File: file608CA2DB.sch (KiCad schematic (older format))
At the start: 1 part, among them SW5 SW_SP3T

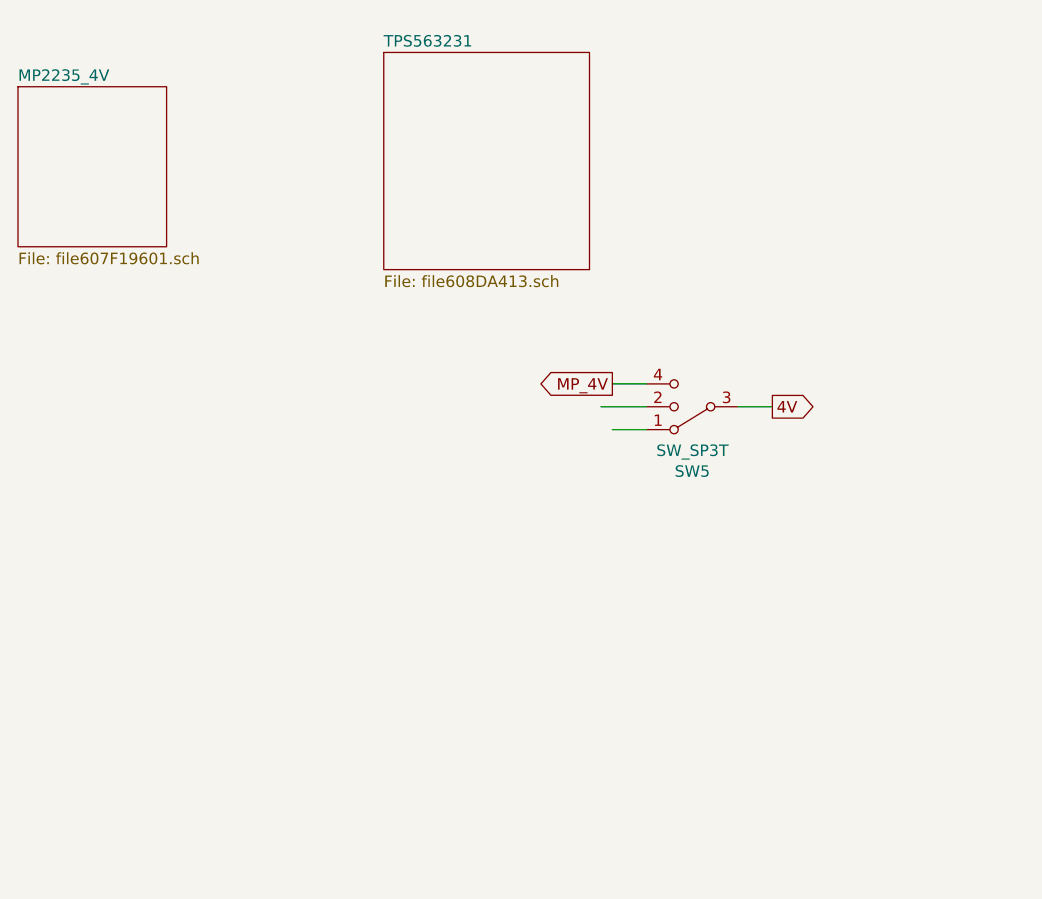
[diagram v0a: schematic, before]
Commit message: full schematic, version 1.0
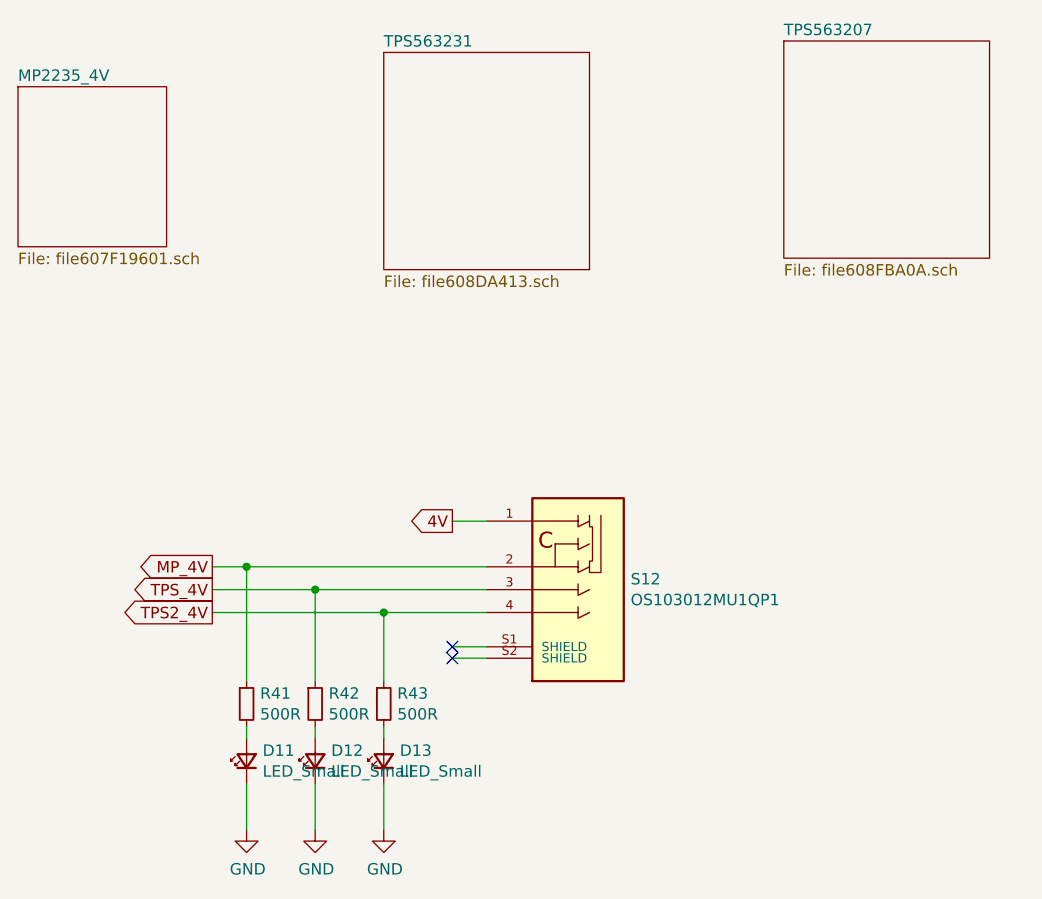
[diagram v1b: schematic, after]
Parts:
- removed SW5: SW_SP3T, symbol Switch:SW_SP3T
- added D11, D12, D13: LED_Small, Diode_SMD:D_0603_1608Metric_Pad1.05x0.95mm_HandSolder, symbol Device:LED_Small
- added R41, R42, R43: 500R, Resistor_SMD:R_0805_2012Metric_Pad1.20x1.40mm_HandSolder, symbol Device:R_Small
- added S12: OS103012MU1QP1, EIPP:SW_OS103012MU1QP1, symbol EIPP_LIBRARY:OS103012MU1QP1
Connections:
- net labels added: GND, TPS2_4V, TPS_4V
- wire segments 4 -> 18
- no-connect marks 0 -> 2
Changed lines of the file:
@@
 $Descr A4 11693 8268
 encoding utf-8
-Sheet 8 10
+Sheet 8 15
 Title ""
 Date ""
@@
 Comment4 ""
 $EndDescr
-$Comp
-L Switch:SW_SP3T SW?
-U 1 1 608CBBC4
-P 5500 3200
-AR Path="/607D64D2/608CBBC4" Ref="SW?"  Part="1"
-AR Path="/608CA2DC/608CBBC4" Ref="SW5"  Part="1"
-F 0 "SW5" H 5500 3483 50  0000 C CNN
-F 1 "SW_SP3T" H 5500 3392 50  0000 C CNN
-F 2 "" H 4875 3375 50  0001 C CNN
-F 3 "~" H 4875 3375 50  0001 C CNN
-	1    5500 3200
-	-1   0    0    1
-$EndComp
-Wire Wire Line
-	5150 3100 5300 3100
-Wire Wire Line
-	5300 3200 5100 3200
-Wire Wire Line
-	5300 3300 5150 3300
-Wire Wire Line
-	5700 3200 5850 3200
-Text GLabel 5850 3200 2    50   Output ~ 0
+Wire Wire Line
+	4600 3700 4450 3700
+Text GLabel 4450 3700 0    50   Output ~ 0
 4V
-Text GLabel 5150 3100 0    50   Output ~ 0
+Text GLabel 3400 3900 0    50   Output ~ 0
 MP_4V
 $Sheet
@@
 F1 "file608DA413.sch" 50
 $EndSheet
+Text GLabel 3400 4000 0    50   Output ~ 0
+TPS_4V
+$Sheet
+S 5900 1600 900  950
+U 608FBA0B
+F0 "TPS563207" 50
+F1 "file608FBA0A.sch" 50
+$EndSheet
+Text GLabel 3400 4100 0    50   Output ~ 0
+TPS2_4V
+$Comp
+L EIPP_LIBRARY:OS103012MU1QP1 S12
+U 1 1 608FBF88
+P 5000 4000
+F 0 "S12" H 5230 4046 50  0000 L CNN
+F 1 "OS103012MU1QP1" H 5230 3955 50  0000 L CNN
+F 2 "EIPP:SW_OS103012MU1QP1" H 5000 4000 50  0001 L BNN
+F 3 "" H 5000 4000 50  0001 L BNN
+F 4 "9.2 mm" H 5000 4000 50  0001 L BNN "MAXIMUM_PACKAGE_HEIGHT"
+F 5 "C and K Switches" H 5000 4000 50  0001 L BNN "MANUFACTURER"
+F 6 "Manufacturer Recommendations" H 5000 4000 50  0001 L BNN "STANDARD"
+F 7 "8 Aug 17" H 5000 4000 50  0001 L BNN "PARTREV"
+	1    5000 4000
+	1    0    0    -1
+$EndComp
+Wire Wire Line
+	4600 4250 4450 4250
+Wire Wire Line
+	4600 4300 4450 4300
+NoConn ~ 4450 4250
+NoConn ~ 4450 4300
+$Comp
+L Device:LED_Small D?
+U 1 1 6082AFB8
+P 3550 4750
+AR Path="/60925CA4/6082AFB8" Ref="D?"  Part="1"
+AR Path="/608CA2DC/6082AFB8" Ref="D11"  Part="1"
+F 0 "D11" V 3596 4680 50  0000 R CNN
+F 1 "LED_Small" V 3505 4680 50  0000 R CNN
+F 2 "Diode_SMD:D_0603_1608Metric_Pad1.05x0.95mm_HandSolder" V 3550 4750 50  0001 C CNN
+F 3 "~" V 3550 4750 50  0001 C CNN
+	1    3550 4750
+	0    -1   -1   0
+$EndComp
+$Comp
+L Device:R_Small R?
+U 1 1 6082AFBE
+P 3550 4500
+AR Path="/60925CA4/6082AFBE" Ref="R?"  Part="1"
+AR Path="/608CA2DC/6082AFBE" Ref="R41"  Part="1"
+F 0 "R41" H 3609 4546 50  0000 L CNN
+F 1 "500R" H 3609 4455 50  0000 L CNN
+F 2 "Resistor_SMD:R_0805_2012Metric_Pad1.20x1.40mm_HandSolder" H 3550 4500 50  0001 C CNN
+F 3 "~" H 3550 4500 50  0001 C CNN
+	1    3550 4500
+	1    0    0    -1
+$EndComp
+Wire Wire Line
+	3550 4650 3550 4600
+Wire Wire Line
+	3550 4400 3550 3900
+Wire Wire Line
+	3550 4850 3550 5050
+$Comp
+L power:GND #PWR?
+U 1 1 6082AFC7
+P 3550 5050
+AR Path="/60925CA4/6082AFC7" Ref="#PWR?"  Part="1"
+AR Path="/608CA2DC/6082AFC7" Ref="#PWR062"  Part="1"
+F 0 "#PWR062" H 3550 4800 50  0001 C CNN
+F 1 "GND" H 3555 4877 50  0000 C CNN
+F 2 "" H 3550 5050 50  0001 C CNN
+F 3 "" H 3550 5050 50  0001 C CNN
+	1    3550 5050
+	1    0    0    -1
+$EndComp
+$Comp
+L Device:LED_Small D?
+U 1 1 6082AFCD
+P 3850 4750
+AR Path="/60925CA4/6082AFCD" Ref="D?"  Part="1"
+AR Path="/608CA2DC/6082AFCD" Ref="D12"  Part="1"
+F 0 "D12" V 3896 4680 50  0000 R CNN
+F 1 "LED_Small" V 3805 4680 50  0000 R CNN
+F 2 "Diode_SMD:D_0603_1608Metric_Pad1.05x0.95mm_HandSolder" V 3850 4750 50  0001 C CNN
+F 3 "~" V 3850 4750 50  0001 C CNN
+	1    3850 4750
+	0    -1   -1   0
+$EndComp
+$Comp
+L Device:R_Small R?
+U 1 1 6082AFD3
+P 3850 4500
+AR Path="/60925CA4/6082AFD3" Ref="R?"  Part="1"
+AR Path="/608CA2DC/6082AFD3" Ref="R42"  Part="1"
+F 0 "R42" H 3909 4546 50  0000 L CNN
+F 1 "500R" H 3909 4455 50  0000 L CNN
+F 2 "Resistor_SMD:R_0805_2012Metric_Pad1.20x1.40mm_HandSolder" H 3850 4500 50  0001 C CNN
+F 3 "~" H 3850 4500 50  0001 C CNN
+	1    3850 4500
+	1    0    0    -1
+$EndComp
+Wire Wire Line
+	3850 4650 3850 4600
+Wire Wire Line
+	3850 4850 3850 5050
+$Comp
+L power:GND #PWR?
+U 1 1 6082AFDB
+P 3850 5050
+AR Path="/60925CA4/6082AFDB" Ref="#PWR?"  Part="1"
+AR Path="/608CA2DC/6082AFDB" Ref="#PWR063"  Part="1"
+F 0 "#PWR063" H 3850 4800 50  0001 C CNN
+F 1 "GND" H 3855 4877 50  0000 C CNN
+F 2 "" H 3850 5050 50  0001 C CNN
+F 3 "" H 3850 5050 50  0001 C CNN
+	1    3850 5050
+	1    0    0    -1
+$EndComp
+$Comp
+L Device:LED_Small D?
+U 1 1 6082AFE1
+P 4150 4750
+AR Path="/60925CA4/6082AFE1" Ref="D?"  Part="1"
+AR Path="/608CA2DC/6082AFE1" Ref="D13"  Part="1"
+F 0 "D13" V 4196 4680 50  0000 R CNN
+F 1 "LED_Small" V 4105 4680 50  0000 R CNN
+F 2 "Diode_SMD:D_0603_1608Metric_Pad1.05x0.95mm_HandSolder" V 4150 4750 50  0001 C CNN
+F 3 "~" V 4150 4750 50  0001 C CNN
+	1    4150 4750
+	0    -1   -1   0
+$EndComp
+$Comp
+L Device:R_Small R?
+U 1 1 6082AFE7
+P 4150 4500
+AR Path="/60925CA4/6082AFE7" Ref="R?"  Part="1"
+AR Path="/608CA2DC/6082AFE7" Ref="R43"  Part="1"
+F 0 "R43" H 4209 4546 50  0000 L CNN
+F 1 "500R" H 4209 4455 50  0000 L CNN
+F 2 "Resistor_SMD:R_0805_2012Metric_Pad1.20x1.40mm_HandSolder" H 4150 4500 50  0001 C CNN
+F 3 "~" H 4150 4500 50  0001 C CNN
+	1    4150 4500
+	1    0    0    -1
+$EndComp
+Wire Wire Line
+	4150 4650 4150 4600
+Wire Wire Line
+	4150 4850 4150 5050
+$Comp
+L power:GND #PWR?
+U 1 1 6082AFEF
+P 4150 5050
+AR Path="/60925CA4/6082AFEF" Ref="#PWR?"  Part="1"
+AR Path="/608CA2DC/6082AFEF" Ref="#PWR064"  Part="1"
+F 0 "#PWR064" H 4150 4800 50  0001 C CNN
+F 1 "GND" H 4155 4877 50  0000 C CNN
+F 2 "" H 4150 5050 50  0001 C CNN
+F 3 "" H 4150 5050 50  0001 C CNN
+	1    4150 5050
+	1    0    0    -1
+$EndComp
+Wire Wire Line
+	3850 4000 3850 4400
+Wire Wire Line
+	4150 4100 4150 4400
+Wire Wire Line
+	4150 4100 4600 4100
+Wire Wire Line
+	3850 4000 4600 4000
+Wire Wire Line
+	4150 4100 3400 4100
+Connection ~ 4150 4100
+Wire Wire Line
+	3400 4000 3850 4000
+Connection ~ 3850 4000
+Wire Wire Line
+	3550 3900 4600 3900
+Wire Wire Line
+	3550 3900 3400 3900
+Connection ~ 3550 3900
 $EndSCHEMATC
